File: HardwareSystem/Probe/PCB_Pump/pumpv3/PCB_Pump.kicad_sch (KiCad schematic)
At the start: 23 parts, among them J1 Conn_01x04_Pin, Q1 IRF510, Q2 IRF4905, U2 MC33063AP, U3 LM7805_TO220

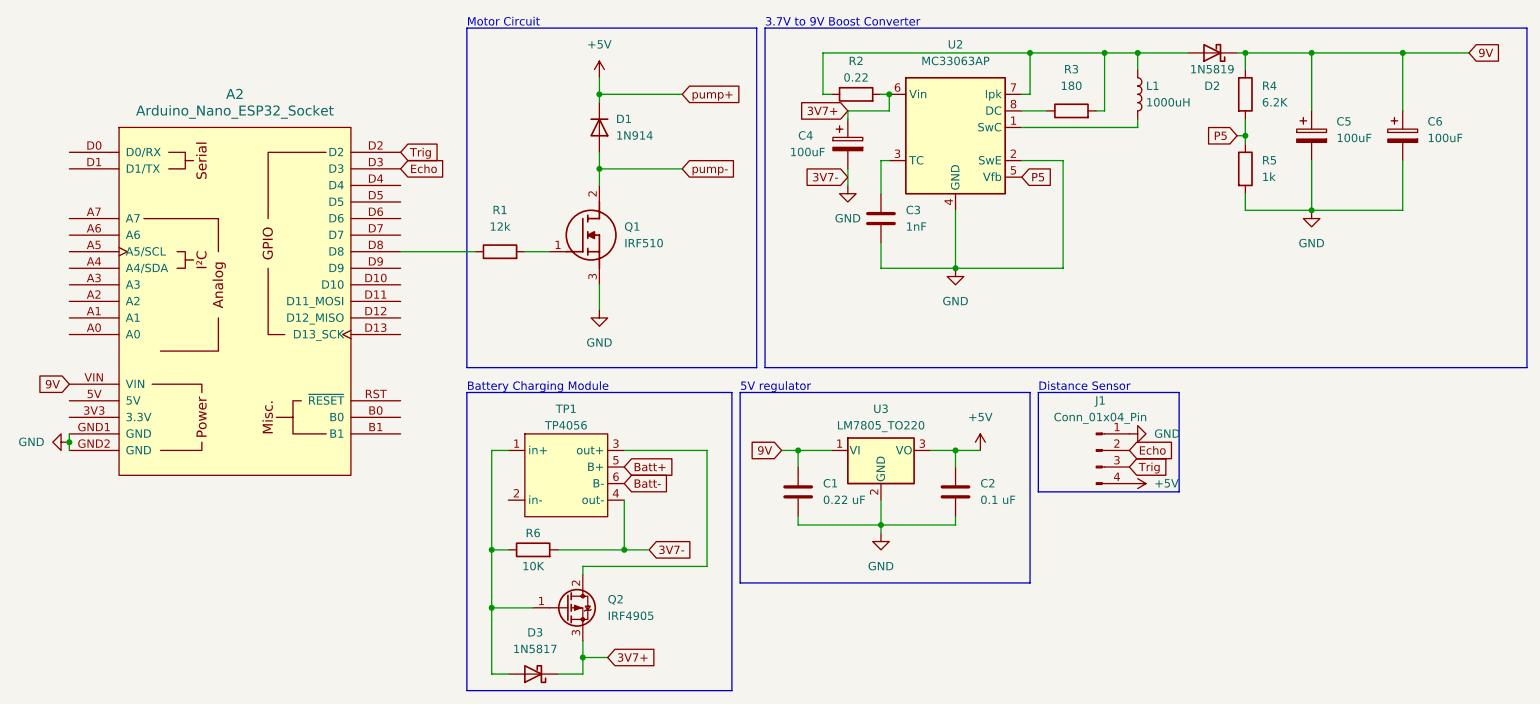
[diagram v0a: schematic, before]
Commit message: updates on both boards
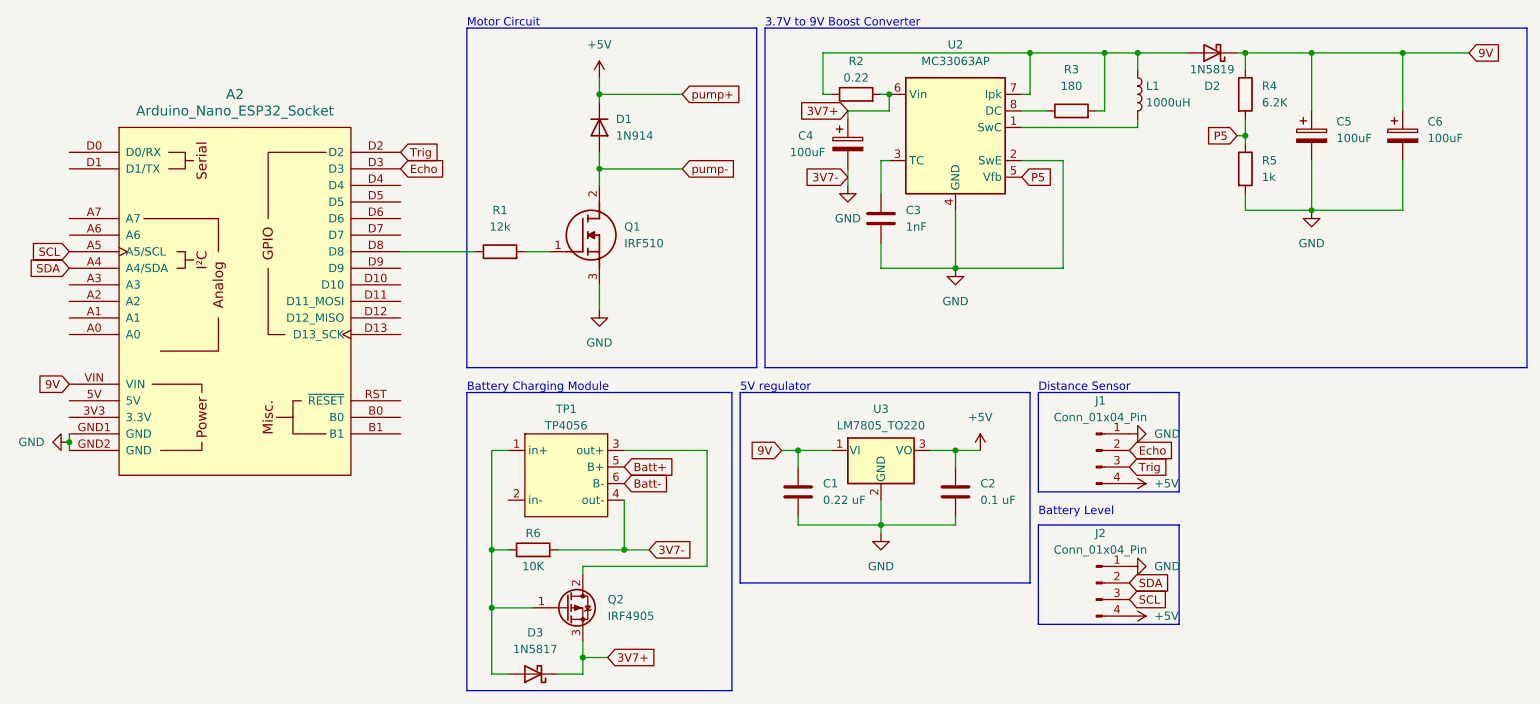
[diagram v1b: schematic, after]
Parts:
- added J2: Conn_01x04_Pin, Connector_PinHeader_2.54mm:PinHeader_1x04_P2.54mm_Vertical, symbol Connector:Conn_01x04_Pin
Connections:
- net +5V: now also J2.4 (Pin_4)
- net GND: now also J2.1 (Pin_1)
- net SDA: now reaches A2.A4 (A4/SDA)
- net SDA: now also J2.2 (Pin_2)
- net SCL: now reaches A2.A5 (A5/SCL)
- net SCL: now also J2.3 (Pin_3)
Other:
- note added: "Battery Level"
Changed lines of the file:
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@@
+    (fill (type none))
+  )
+  (rectangle (start 175.26 99.06) (end 196.85 114.3)
+    (stroke (width 0) (type default))
     (fill (type none))
   )
@@
   )
   (text "Battery Charging Module" (at 87.63 78.74 0)
+    (effects (font (size 1.27 1.27)) (justify left bottom))
+  )
+  (text "Battery Level" (at 175.26 97.79 0)
     (effects (font (size 1.27 1.27)) (justify left bottom))
   )
@@
     )
   )
+  (global_label "SCL" (shape input) (at 189.23 110.49 0) (fields_autoplaced)
+    (effects (font (size 1.27 1.27)) (justify left))
+    (property "Intersheetrefs" "${INTERSHEET_REFS}" (at 195.7228 110.49 0)
+      (effects (font (size 1.27 1.27)) (justify left) hide)
+    )
+  )
   (global_label "3V7-" (shape input) (at 146.05 45.72 180) (fields_autoplaced)
     (effects (font (size 1.27 1.27)) (justify right))
@@
     )
   )
+  (global_label "SCL" (shape input) (at 26.67 57.15 180) (fields_autoplaced)
+    (effects (font (size 1.27 1.27)) (justify right))
+    (property "Intersheetrefs" "${INTERSHEET_REFS}" (at 20.1772 57.15 0)
+      (effects (font (size 1.27 1.27)) (justify right) hide)
+    )
+  )
   (global_label "Echo" (shape input) (at 189.23 87.63 0) (fields_autoplaced)
     (effects (font (size 1.27 1.27)) (justify left))
@@
     (effects (font (size 1.27 1.27)) (justify left))
     (property "Intersheetrefs" "${INTERSHEET_REFS}" (at 178.1847 45.72 0)
+      (effects (font (size 1.27 1.27)) (justify left) hide)
+    )
+  )
+  (global_label "SDA" (shape input) (at 26.67 59.69 180) (fields_autoplaced)
+    (effects (font (size 1.27 1.27)) (justify right))
+    (property "Intersheetrefs" "${INTERSHEET_REFS}" (at 20.1167 59.69 0)
+      (effects (font (size 1.27 1.27)) (justify right) hide)
+    )
+  )
+  (global_label "SDA" (shape input) (at 189.23 107.95 0) (fields_autoplaced)
+    (effects (font (size 1.27 1.27)) (justify left))
+    (property "Intersheetrefs" "${INTERSHEET_REFS}" (at 195.7833 107.95 0)
       (effects (font (size 1.27 1.27)) (justify left) hide)
     )
@@
         (path "/57512134-c0e5-4e7f-86c3-2738c5b8ae18"
           (reference "C2") (unit 1)
+        )
+      )
+    )
+  )
+  (symbol (lib_id "Connector:Conn_01x04_Pin") (at 184.15 107.95 0) (unit 1)
+    (in_bom yes) (on_board yes) (dnp no) (fields_autoplaced)
+    (property "Reference" "J2" (at 184.785 100.33 0)
+      (effects (font (size 1.27 1.27)))
+    )
+    (property "Value" "Conn_01x04_Pin" (at 184.785 102.87 0)
+      (effects (font (size 1.27 1.27)))
+    )
+    (property "Footprint" "Connector_PinHeader_2.54mm:PinHeader_1x04_P2.54mm_Vertical" (at 184.15 107.95 0)
+      (effects (font (size 1.27 1.27)) hide)
+    )
+    (property "Datasheet" "~" (at 184.15 107.95 0)
+      (effects (font (size 1.27 1.27)) hide)
+    )
+    (pin "1")
+    (pin "2")
+    (pin "3")
+    (pin "4")
+    (instances
+      (project "PCB_Pump"
+        (path "/57512134-c0e5-4e7f-86c3-2738c5b8ae18"
+          (reference "J2") (unit 1)
         )
       )
@@
     )
   )
+  (symbol (lib_id "power:+5V") (at 189.23 113.03 270) (unit 1)
+    (in_bom yes) (on_board yes) (dnp no) (fields_autoplaced)
+    (property "Reference" "#PWR011" (at 185.42 113.03 0)
+      (effects (font (size 1.27 1.27)) hide)
+    )
+    (property "Value" "+5V" (at 193.04 113.03 90)
+      (effects (font (size 1.27 1.27)) (justify left))
+    )
+    (property "Footprint" "" (at 189.23 113.03 0)
+      (effects (font (size 1.27 1.27)) hide)
+    )
+    (property "Datasheet" "" (at 189.23 113.03 0)
+      (effects (font (size 1.27 1.27)) hide)
+    )
+    (pin "1")
+    (instances
+      (project "PCB_Pump"
+        (path "/57512134-c0e5-4e7f-86c3-2738c5b8ae18"
+          (reference "#PWR011") (unit 1)
+        )
+      )
+    )
+  )
   (symbol (lib_id "Diode:1N5819") (at 201.93 26.67 180) (unit 1)
     (in_bom yes) (on_board yes) (dnp no)
@@
         )
       )
+    )
+  )
+  (symbol (lib_id "power:GND") (at 189.23 105.41 90) (unit 1)
+    (in_bom yes) (on_board yes) (dnp no) (fields_autoplaced)
+    (property "Reference" "#PWR012" (at 195.58 105.41 0)
+      (effects (font (size 1.27 1.27)) hide)
+    )
+    (property "Value" "GND" (at 193.04 105.41 90)
+      (effects (font (size 1.27 1.27)) (justify right))
+    )
+    (property "Footprint" "" (at 189.23 105.41 0)
+      (effects (font (size 1.27 1.27)) hide)
+    )
+    (property "Datasheet" "" (at 189.23 105.41 0)
+      (effects (font (size 1.27 1.27)) hide)
+    )
+    (pin "1")
+    (instances
+      (project "PCB_Pump"
+        (path "/57512134-c0e5-4e7f-86c3-2738c5b8ae18"
+          (reference "#PWR012") (unit 1)
+        )
+      )
